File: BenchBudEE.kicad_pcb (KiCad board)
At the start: 4 copper layers, 165.1 x 63.5 mm, 107 parts, among them K1 RELAY, P1 24 Pin MiniFit JR, P2 CONN_2, P3 CONN_3X2, P4 12 Pin Terminal Block, P5 CONN_3, Q1 2N3904, Q2 MOSFET_N, Q3 NMOS, Q4 NMOS, SW1 SWITCH, U1 OPTO_TRANSISTOR, U10 LM317, U2 MCP3901, U3 LMT84, U4 OPA4170, U5 AP5726, U6 MCP4801, U7 LM337T, U8 LM317, U9 LM337T

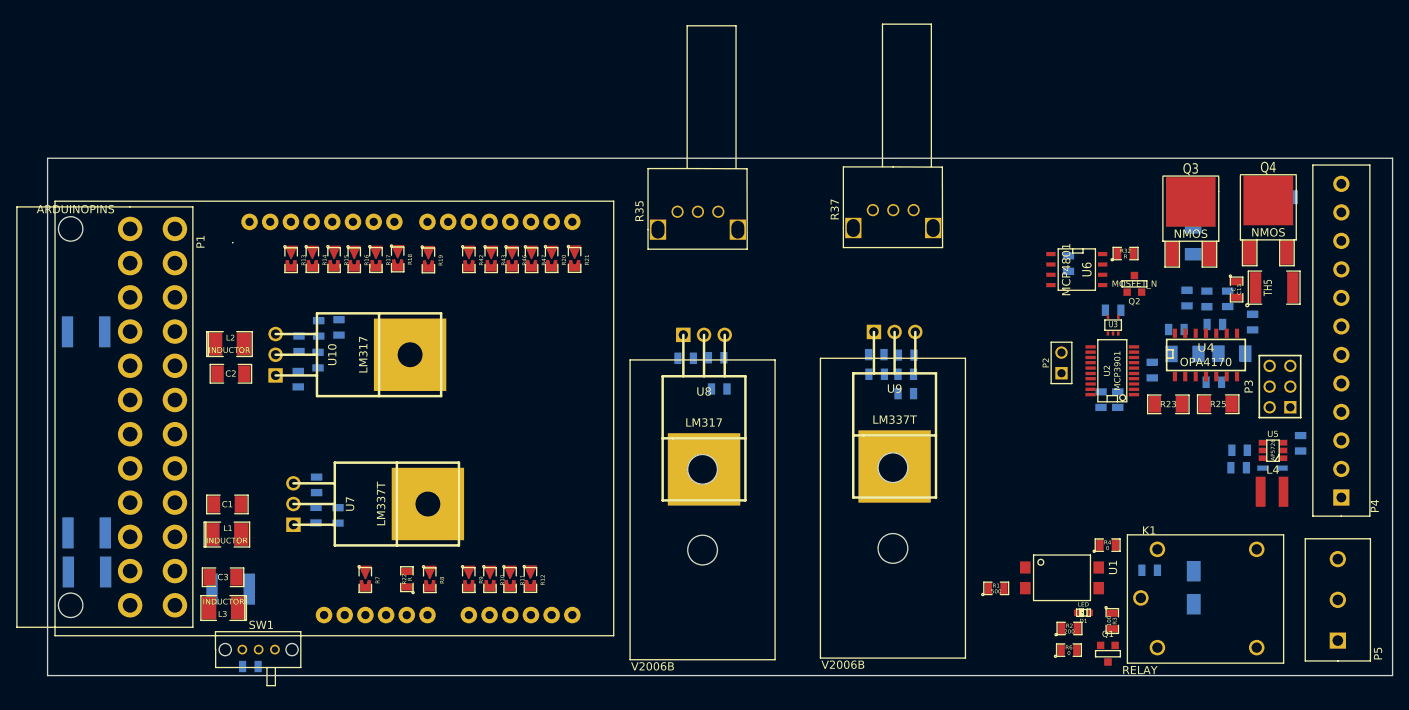
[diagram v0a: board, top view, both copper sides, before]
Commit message: Layout v1.0
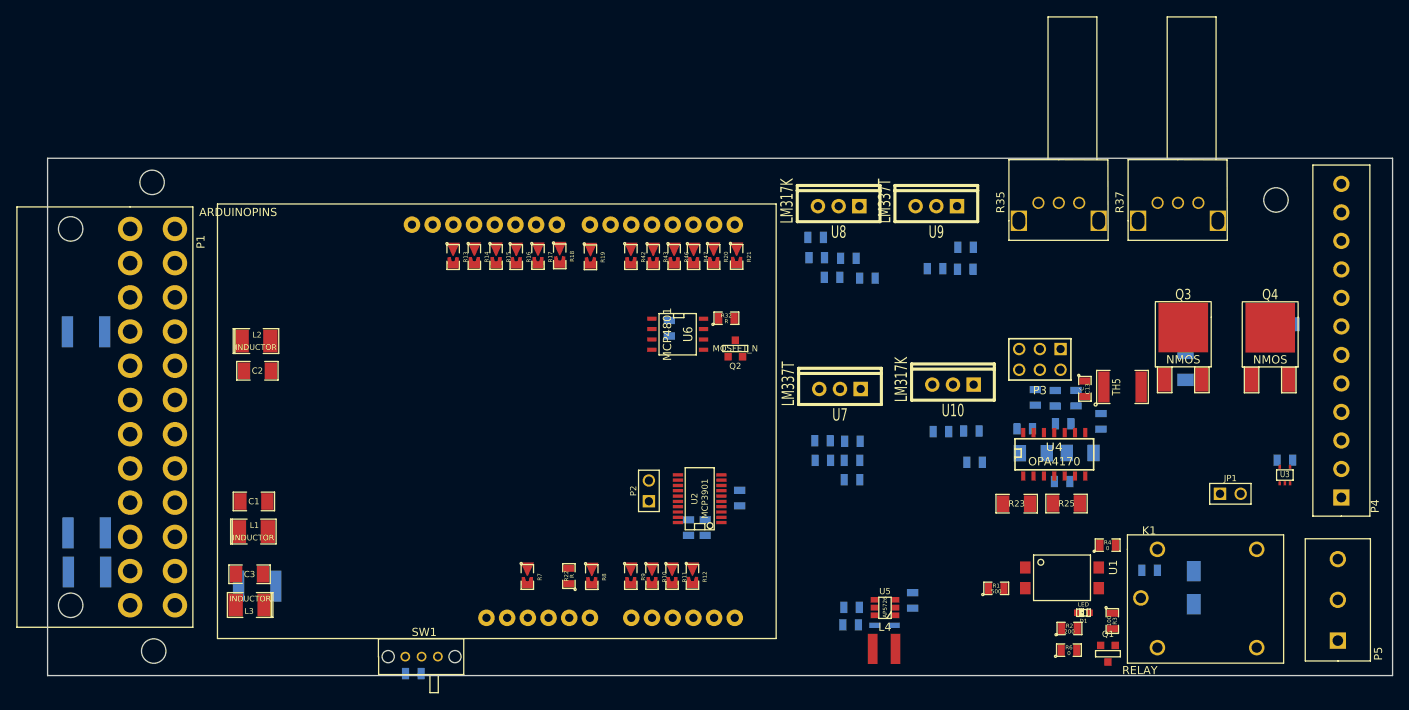
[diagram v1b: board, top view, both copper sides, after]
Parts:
- removed V2006B (x2): VAL**, V2006B
- added 3mm_drill: VAL**, 3mm_drill, F.Cu at (80.1, 124.1)
- added 3mm_drill: VAL**, 3mm_drill, F.Cu at (80.3, 181.6)
- added 3mm_drill: VAL**, 3mm_drill, F.Cu at (218.1, 126.2)
- added JP1: JUMPER, PIN_ARRAY_2X1, F.Cu at (212.5, 162.3)
- U10, U8: value LM317 -> LM317K; footprint TO220 -> TO220_VERT
- U7, U9: footprint TO220 -> TO220_VERT
- moved R49 85.2 mm to (179.9, 134.7), turned to 0 degrees
- moved R48 83.8 mm to (180.0, 132.0), turned to 180 degrees
- moved U10 83.2 mm to (178.4, 148.9), turned to 90 degrees
- moved C16 80.4 mm to (176.2, 134.7), turned to 0 degrees
- moved C15 71.0 mm to (167.9, 135.8), turned to 0 degrees
- moved U7 68.6 mm to (164.6, 149.4), turned to 90 degrees
- moved C17 66.3 mm to (165.6, 133.4), turned to 0 degrees
- moved R50 65.9 mm to (163.6, 135.7), turned to 180 degrees
- moved R51 61.8 mm to (161.7, 133.3), turned to 180 degrees
- moved R39 59.6 mm to (161.6, 130.8), turned to 180 degrees
- moved C6 53.0 mm to (148.0, 166.5)
- moved C7 53.0 mm to (146.0, 166.5)
- moved U2 53.0 mm to (147.3, 162.9)
- moved P2 53.0 mm to (141.1, 162.0)
- moved C8 53.0 mm to (152.2, 162.8)
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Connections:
- C13 pad 2: AGND -> GND
- K1 pad 3: /Relay/RELAY_NO -> /Relay/RELAY_NC
- K1 pad 4: /Relay/RELAY_NC -> /Relay/RELAY_NO
- Q3 pad 3: AGND -> GND
- R33 pad 2: AGND -> GND
- R34 pad 2: N-00000118 (its old number) -> N-00000120
- R35 pad 1: N-00000118 (its old number) -> N-00000120
- R50 pad 2: N-00000122 -> N-00000121
- R51 pad 1: N-00000122 -> N-00000121
- TH1 pad 2: (no net) -> +3.3V
- U10 pad 1: +12V -> N-00000120
- U10 pad 2: N-00000122 -> +12V
- U10 pad 3: FE_V+ -> /Power_Adjustment_Monitor/V+_ADJ
- U4 pad 11: -12V -> FE_V-
- U4 pad 4: +12V -> FE_V+
- U8 pad 1: +12V -> N-00000121
- U8 pad 2: N-00000118 (its old number) -> +12V
- U8 pad 3: /Power_Adjustment_Monitor/V+_ADJ -> FE_V+
- U9 pad 2: /Power_Adjustment_Monitor/V-_ADJ -> -12V
- U9 pad 3: -12V -> /Power_Adjustment_Monitor/V-_ADJ
